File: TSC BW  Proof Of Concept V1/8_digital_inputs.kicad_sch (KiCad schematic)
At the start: 38 parts, among them J5 Terminal Plug, U10 PC357C, U11 PC357C, U14 PC357C, U15 PC357C, U18 PC357C, U19 PC357C, U20 PCF8574T, U6 PC357C, U7 PC357C

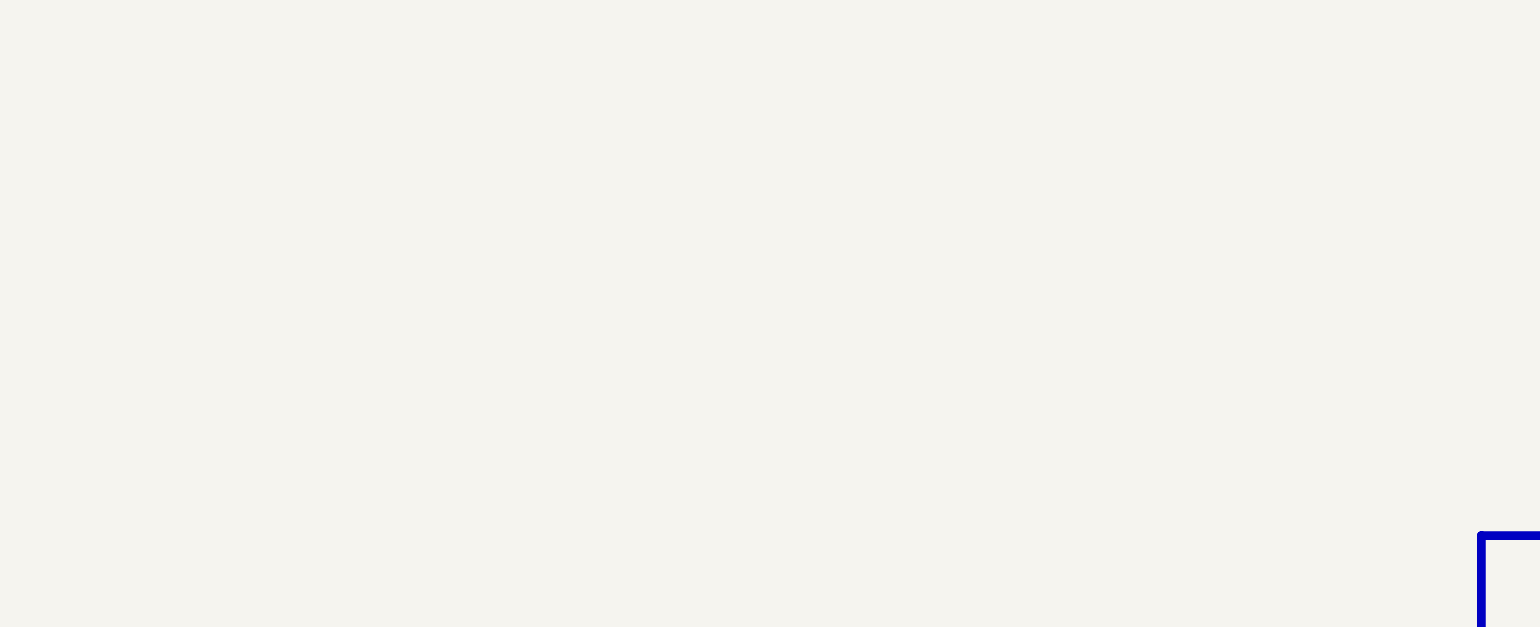
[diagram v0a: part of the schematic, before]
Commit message: WORKING ON POC - Proof of concept
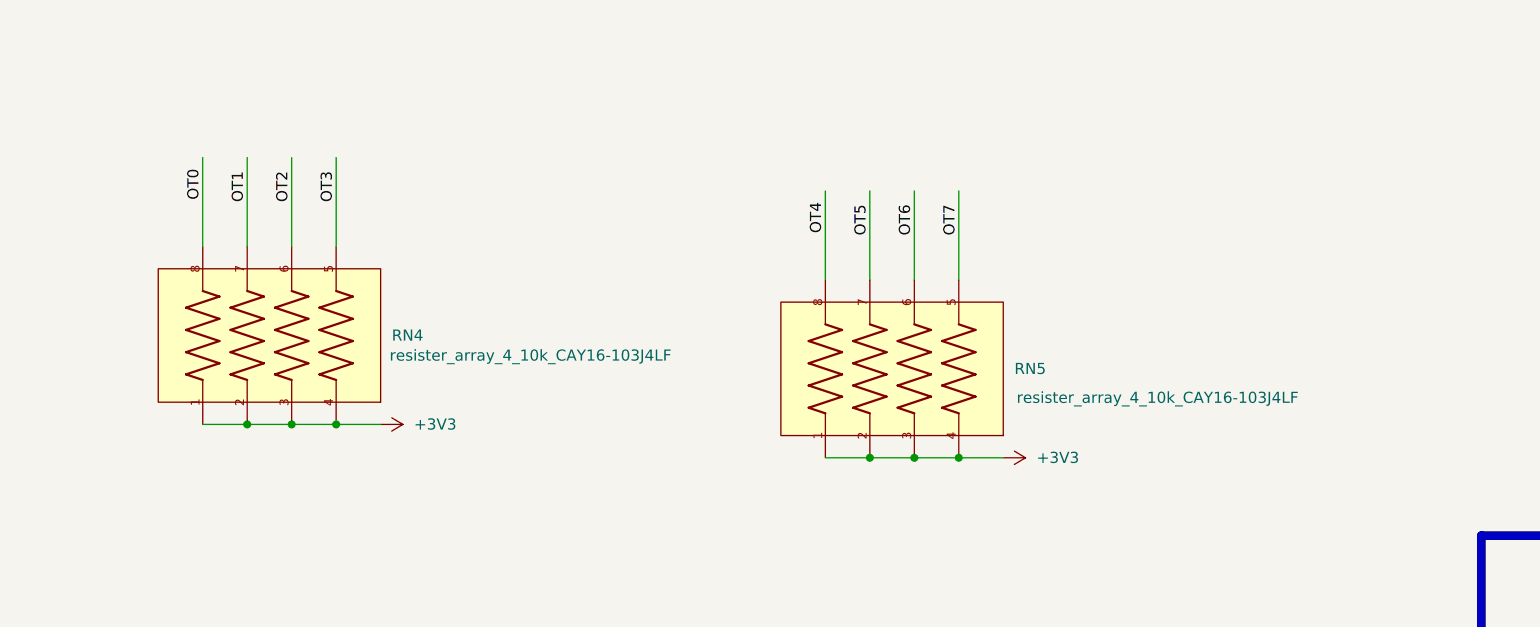
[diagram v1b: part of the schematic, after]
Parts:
- added RN4, RN5: resister_array_4_10k_CAY16-103J4LF, Resistor_SMD:R_Array_Convex_4x1206, symbol CAY16-103J4LF:resister_array_4_10k_CAY16-103J4LF
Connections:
- net +3V3: now also RN4.1, RN4.2, RN4.3, RN4.4, RN5.1, RN5.2, RN5.3, RN5.4
- new net OT0: RN4.8
- new net OT1: RN4.7
- new net OT2: RN4.6
- new net OT3: RN4.5
- new net OT4: RN5.8
- new net OT5: RN5.7
- new net OT6: RN5.6
- new net OT7: RN5.5

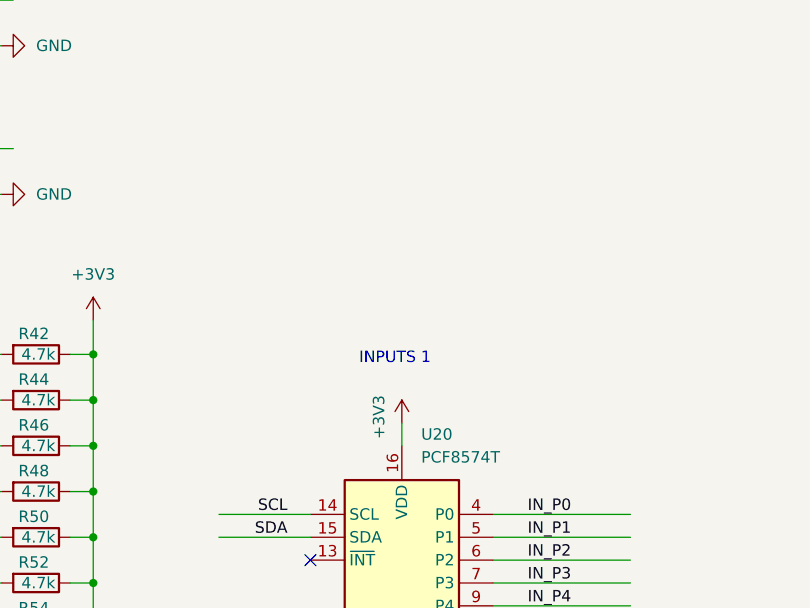
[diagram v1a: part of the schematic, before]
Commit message: WORKING ON POC - Proof of concept
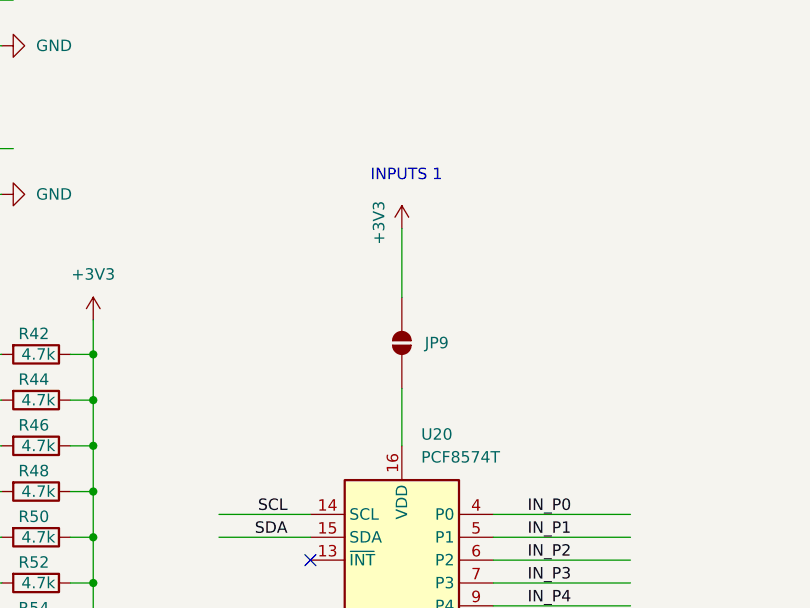
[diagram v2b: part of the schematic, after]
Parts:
- added JP9: SolderJumper_2_Open, Jumper:SolderJumper-2_P1.3mm_Open_RoundedPad1.0x1.5mm, symbol Jumper:SolderJumper_2_Open
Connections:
- net +3V3: now also JP9.1 (A); no longer U20.16 (VDD)
- new net: JP9.2 (B), U20.16 (VDD)
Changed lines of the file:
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@@
 	(text "INPUTS 1"
 		(exclude_from_sim no)
-		(at 133.858 146.558 0)
+		(at 135.128 126.238 0)
 		(effects
 			(font
@@
 	(wire
 		(pts
-			(xy 134.62 153.67) (xy 134.62 156.21)
+			(xy 134.62 132.08) (xy 134.62 139.7)
 		)
 		(stroke
@@
 	(wire
 		(pts
+			(xy 134.62 149.86) (xy 134.62 156.21)
+		)
+		(stroke
+			(width 0)
+			(type default)
+		)
+	)
+	(wire
+		(pts
 			(xy 209.55 184.15) (xy 214.63 184.15)
 		)
@@
 	)
 	(symbol
+		(lib_id "Jumper:SolderJumper_2_Open")
+		(at 134.62 144.78 270)
+		(unit 1)
+		(body_style 1)
+		(exclude_from_sim no)
+		(in_bom no)
+		(on_board yes)
+		(in_pos_files yes)
+		(dnp no)
+		(fields_autoplaced yes)
+		(property "Reference" "JP9"
+			(at 137.16 144.7799 90)
+			(show_name no)
+			(do_not_autoplace no)
+			(effects
+				(font
+					(size 1.27 1.27)
+				)
+				(justify left)
+			)
+		)
+		(property "Value" "SolderJumper_2_Open"
+			(at 138.43 144.78 0)
+			(hide yes)
+			(show_name no)
+			(do_not_autoplace no)
+			(effects
+				(font
+					(size 1.27 1.27)
+				)
+			)
+		)
+		(property "Footprint" "Jumper:SolderJumper-2_P1.3mm_Open_RoundedPad1.0x1.5mm"
+			(at 134.62 144.78 0)
+			(hide yes)
+			(show_name no)
+			(do_not_autoplace no)
+			(effects
+				(font
+					(size 1.27 1.27)
+				)
+			)
+		)
+		(property "Datasheet" ""
+			(at 127 144.78 0)
+			(hide yes)
+			(show_name no)
+			(do_not_autoplace no)
+			(effects
+				(font
+					(size 1.27 1.27)
+				)
+			)
+		)
+		(property "Description" "Solder Jumper, 2-pole, open"
+			(at 129.54 144.78 0)
+			(hide yes)
+			(show_name no)
+			(do_not_autoplace no)
+			(effects
+				(font
+					(size 1.27 1.27)
+				)
+			)
+		)
+		(pin "2"
+		)
+		(pin "1"
+		)
+		(instances
+			(project "TSC BW 16 V3 POC"
+				(path "/65a0f6c1-6a57-4cd2-a77c-79691e6171da/46fc40ab-03f2-48e3-952c-a0230bfbcd31"
+					(reference "JP9")
+					(unit 1)
+				)
+			)
+		)
+	)
+	(symbol
 		(lib_id "power:GND")
 		(at 134.62 215.9 0)
@@
 	(symbol
 		(lib_id "power:+3V3")
-		(at 134.62 153.67 0)
+		(at 134.62 132.08 0)
 		(unit 1)
 		(body_style 1)
@@
 		(dnp no)
 		(property "Reference" "#PWR067"
-			(at 134.62 157.48 0)
+			(at 134.62 135.89 0)
 			(hide yes)
 			(show_name no)
@@
 		)
 		(property "Value" "+3V3"
-			(at 132.08 155.448 90)
+			(at 132.08 133.858 90)
 			(show_name no)
 			(do_not_autoplace no)
@@
 		)
 		(property "Footprint" ""
-			(at 134.62 153.67 0)
+			(at 134.62 132.08 0)
 			(hide yes)
 			(show_name no)
@@
 		)
 		(property "Datasheet" ""
-			(at 134.62 153.67 0)
+			(at 134.62 132.08 0)
 			(hide yes)
 			(show_name no)
@@
 		)
 		(property "Description" "Power symbol creates a global label with name \"+3V3\""
-			(at 134.62 153.67 0)
+			(at 134.62 132.08 0)
 			(hide yes)
 			(show_name no)
